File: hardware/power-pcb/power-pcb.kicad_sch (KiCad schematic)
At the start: 52 parts, among them J1 XT60-M-AS, J13 MicroFit2x12_Odd_Even, J18 Conn_02x07_Odd_Even, J2 XT30, J5 XT30, J6 XT30, J7 XT30, J8 JST_XH_5, Q1 SQJ138EP-T1_GE3, Q2 SQJ138EP-T1_GE3, U1 BTS50010-1TAE, U2 LTC4365TS8, U3 R-78E3.3-1.0, U8 ADS1015IDGS

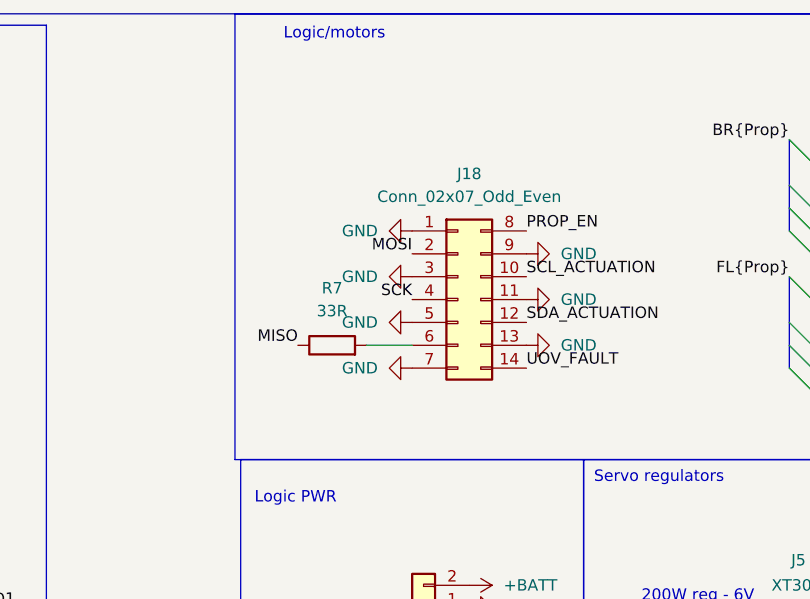
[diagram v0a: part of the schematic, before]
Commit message: fixes pre-prod
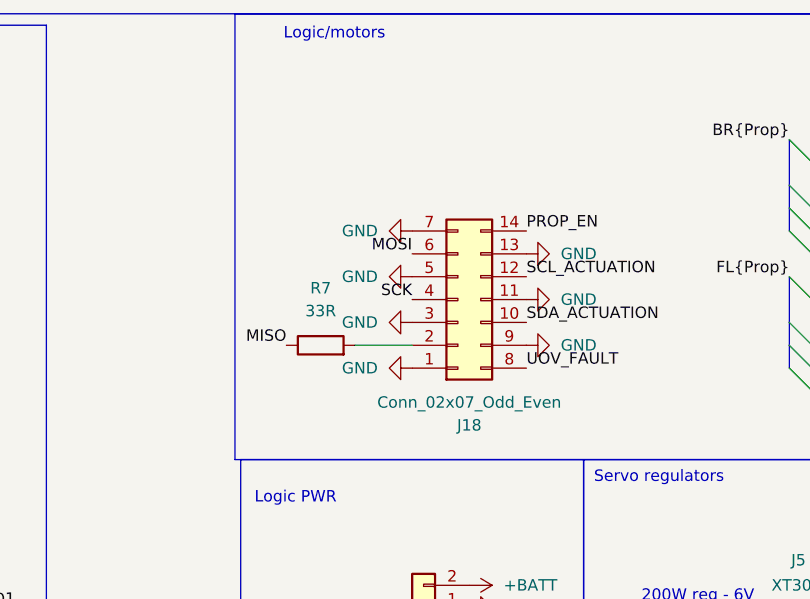
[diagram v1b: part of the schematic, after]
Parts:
- J13: MPN 66202421122 -> 43045-2412; Manufacturer Wurth -> Molex
- J18: MPN 66201421122 -> 43045-1412; Manufacturer Wurth -> Molex
- J2, J5, J6, J7: footprint Project:AMASS_XT30UPB-M_1x02_P5.0mm_Vertical -> Project:AMASS_XT30U-M_1x02_P5.0mm_Vertical
- R2, R41: MPN CRCW0805100K0FKEA -> CRCW0805100KFKEA
- R46: MPN CRCW0805143K0FKEA -> CRCW0805143KFKEA
- R7: MPN CRCW080533RFKEA -> CRCW080533R0FKEA
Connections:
- net MOSI: now also J18.6 (Pin_6); no longer J18.2 (Pin_2)
- net PROP_EN: now also J18.14 (Pin_14); no longer J18.8 (Pin_8)
- net SCL_ACTUATION: now also J18.12 (Pin_12); no longer J18.10 (Pin_10)
- net SDA_ACTUATION: now also J18.10 (Pin_10); no longer J18.12 (Pin_12)
- net UOV_FAULT: now also J18.8 (Pin_8); no longer J18.14 (Pin_14)
- net at R7.2: now also J18.2 (Pin_2); no longer J18.6 (Pin_6)
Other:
- moved on the sheet: R7
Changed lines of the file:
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@@
 	(wire
 		(pts
-			(xy 176.53 106.68) (xy 181.61 106.68)
+			(xy 175.26 106.68) (xy 181.61 106.68)
 		)
 		(stroke
@@
 	)
 	(label "MISO"
-		(at 168.91 106.68 180)
+		(at 167.64 106.68 180)
 		(effects
 			(font
@@
 			)
 		)
-		(property "MPN" "CRCW0805143K0FKEA"
+		(property "MPN" "CRCW0805143KFKEA"
 			(at 120.65 223.52 0)
 			(effects
@@
 			)
 		)
-		(property "MPN" "66202421122"
+		(property "MPN" "43045-2412"
 			(at 245.11 99.06 0)
 			(effects
@@
 			)
 		)
-		(property "Manufacturer" "Wurth"
+		(property "Manufacturer" "Molex"
 			(at 245.11 99.06 0)
 			(effects
@@
 			)
 		)
-		(property "Footprint" "Project:AMASS_XT30UPB-M_1x02_P5.0mm_Vertical"
+		(property "Footprint" "Project:AMASS_XT30U-M_1x02_P5.0mm_Vertical"
 			(at 228.6 130.81 0)
 			(effects
@@
 			)
 		)
-		(property "Footprint" "Project:AMASS_XT30UPB-M_1x02_P5.0mm_Vertical"
+		(property "Footprint" "Project:AMASS_XT30U-M_1x02_P5.0mm_Vertical"
 			(at 182.88 135.89 0)
 			(effects
@@
 			)
 		)
-		(property "MPN" "CRCW0805100K0FKEA"
+		(property "MPN" "CRCW0805100KFKEA"
 			(at 96.52 222.25 0)
 			(effects
@@
 	(symbol
 		(lib_id "Device:R")
-		(at 172.72 106.68 90)
+		(at 171.45 106.68 90)
 		(unit 1)
 		(exclude_from_sim no)
@@
 		(fields_autoplaced yes)
 		(property "Reference" "R7"
-			(at 172.72 100.33 90)
+			(at 171.45 100.33 90)
 			(effects
 				(font
@@
 		)
 		(property "Value" "33R"
-			(at 172.72 102.87 90)
+			(at 171.45 102.87 90)
 			(effects
 				(font
@@
 		)
 		(property "Footprint" "Resistor_SMD:R_0805_2012Metric_Pad1.20x1.40mm_HandSolder"
-			(at 172.72 108.458 90)
+			(at 171.45 108.458 90)
 			(effects
 				(font
@@
 		)
 		(property "Datasheet" "~"
-			(at 172.72 106.68 0)
+			(at 171.45 106.68 0)
 			(effects
 				(font
@@
 		)
 		(property "Description" "Resistor"
-			(at 172.72 106.68 0)
+			(at 171.45 106.68 0)
 			(effects
 				(font
@@
 			)
 		)
-		(property "MPN" "CRCW080533RFKEA"
-			(at 172.72 106.68 90)
+		(property "MPN" "CRCW080533R0FKEA"
+			(at 171.45 106.68 90)
 			(effects
 				(font
@@
 		)
 		(property "Manufacturer" "Vishay"
-			(at 172.72 106.68 90)
+			(at 171.45 106.68 90)
 			(effects
 				(font
@@
 			)
 		)
-		(property "Footprint" "Project:AMASS_XT30UPB-M_1x02_P5.0mm_Vertical"
+		(property "Footprint" "Project:AMASS_XT30U-M_1x02_P5.0mm_Vertical"
 			(at 255.27 130.81 0)
 			(effects
@@
 		(lib_id "Connector_Generic:Conn_02x07_Top_Bottom")
 		(at 186.69 101.6 0)
+		(mirror x)
 		(unit 1)
 		(exclude_from_sim no)
@@
 		(on_board yes)
 		(dnp no)
-		(fields_autoplaced yes)
 		(property "Reference" "J18"
-			(at 187.96 87.63 0)
+			(at 187.96 115.57 0)
 			(effects
 				(font
@@
 		)
 		(property "Value" "Conn_02x07_Odd_Even"
-			(at 187.96 90.17 0)
+			(at 187.96 113.03 0)
 			(effects
 				(font
@@
 			)
 		)
-		(property "MPN" "66201421122"
+		(property "MPN" "43045-1412"
 			(at 186.69 101.6 0)
 			(effects
@@
 			)
 		)
-		(property "Manufacturer" "Wurth"
+		(property "Manufacturer" "Molex"
 			(at 186.69 101.6 0)
 			(effects
@@
 			)
 		)
-		(property "Footprint" "Project:AMASS_XT30UPB-M_1x02_P5.0mm_Vertical"
+		(property "Footprint" "Project:AMASS_XT30U-M_1x02_P5.0mm_Vertical"
 			(at 196.85 46.99 0)
 			(effects
@@
 			)
 		)
-		(property "MPN" "CRCW0805100K0FKEA"
+		(property "MPN" "CRCW0805100KFKEA"
 			(at 110.49 43.18 90)
 			(effects
